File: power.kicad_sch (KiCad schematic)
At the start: 77 parts, among them CON2 BARREL_JACK, U17 LMR51420, U18 LMR51420, U19 LMR51420, U20 LP5907-3.0, U21 LP2985A-10DBVR, U22 LD3920, U23 LD3920, U24 LD3920, U25 BU33SD5WG

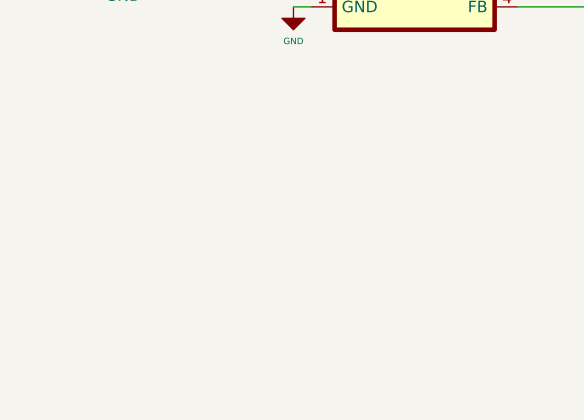
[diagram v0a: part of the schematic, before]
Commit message: hardware changes
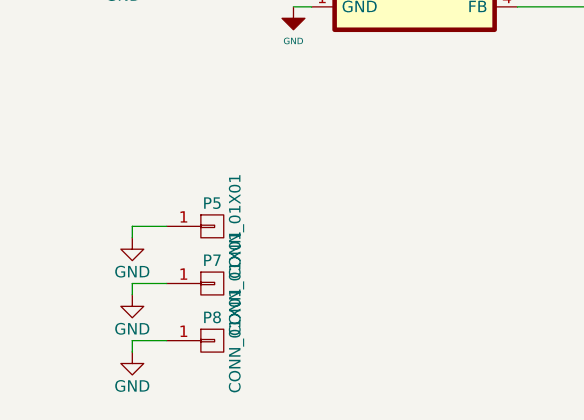
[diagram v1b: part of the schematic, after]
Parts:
- added P5, P7, P8: CONN_01X01, fmcw3:MountingHole_3.2mm_M3_Pad_Via_mod, symbol fmcw3-rescue:CONN_01X01
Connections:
- net GND: now also P5.1 (P1), P7.1 (P1), P8.1 (P1)
